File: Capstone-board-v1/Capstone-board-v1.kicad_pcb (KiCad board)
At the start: 2 copper layers, 53.3 x 45.7 mm, 21 parts, among them J1 Pico Socket 1, J2 Pico Socket 2, J3 Gyroscope Sensor, M1 DC Vibration Motor, Q1 2N3904, U1 3.3 V Voltage Regulator, U2 555 Timer, U3 Hall Effect Sensor, U4 OP Amp

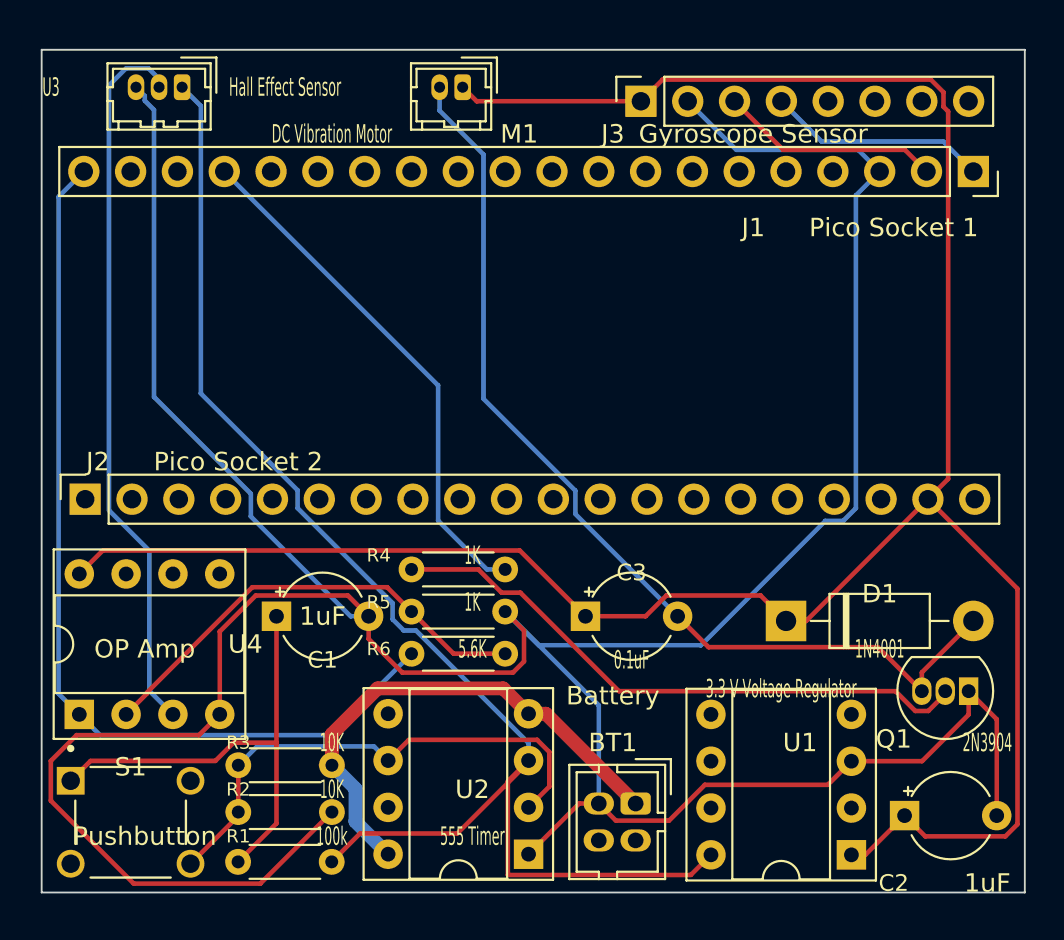
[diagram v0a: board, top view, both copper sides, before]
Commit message: Final PCB completed!
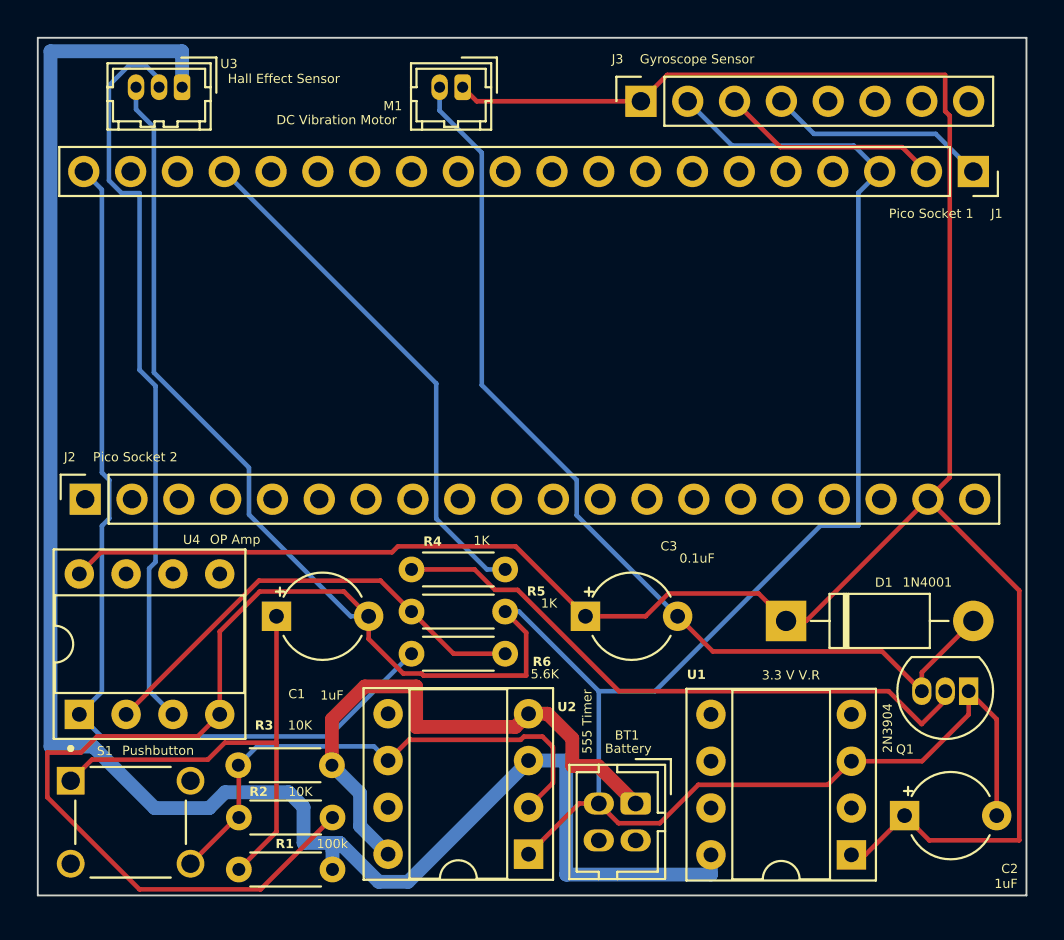
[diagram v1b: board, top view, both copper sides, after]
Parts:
- U1: value 3.3 V Voltage Regulator -> 3.3 V V.R
- moved R1 0.42 mm to (33.0, 65.3)
- moved R2 0.30 mm to (38.1, 62.5)
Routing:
- net Net-(U1-IN): track 75.9 -> 99.4 mm
- net VCC: track 28.5 -> 31.2 mm
- net Net-(D1-K): track 131.9 -> 133.9 mm
- net Earth: track 195.9 -> 193.9 mm
- net Net-(U3-VOUT): track 39.8 -> 40.8 mm
- net Net-(U2-THR): track 28.8 -> 29.7 mm
- net Net-(Q1-B): track 32.7 -> 33.5 mm
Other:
- board size 53.3 x 45.7 mm -> 53.6 x 46.5 mm
